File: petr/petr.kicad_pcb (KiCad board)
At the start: 2 copper layers, 38.5 x 53.6 mm, 4 parts

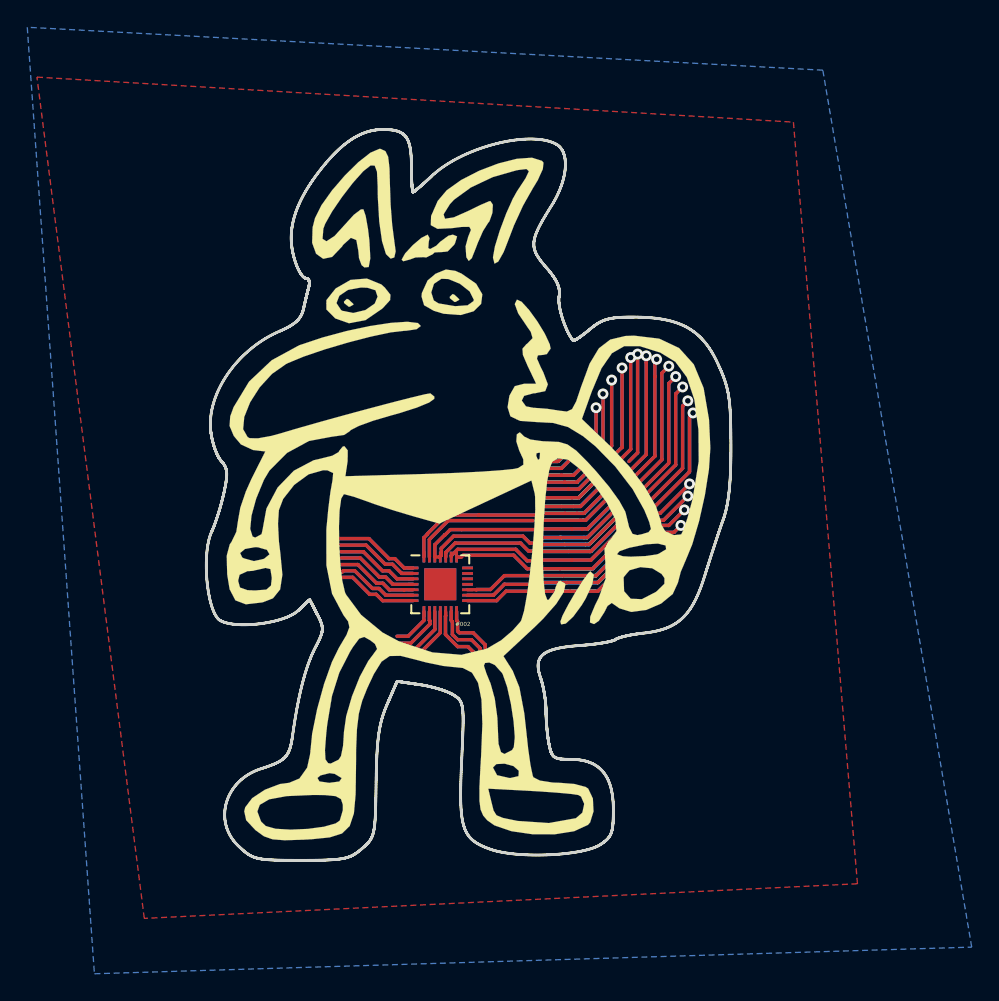
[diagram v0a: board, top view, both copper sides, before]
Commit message: update
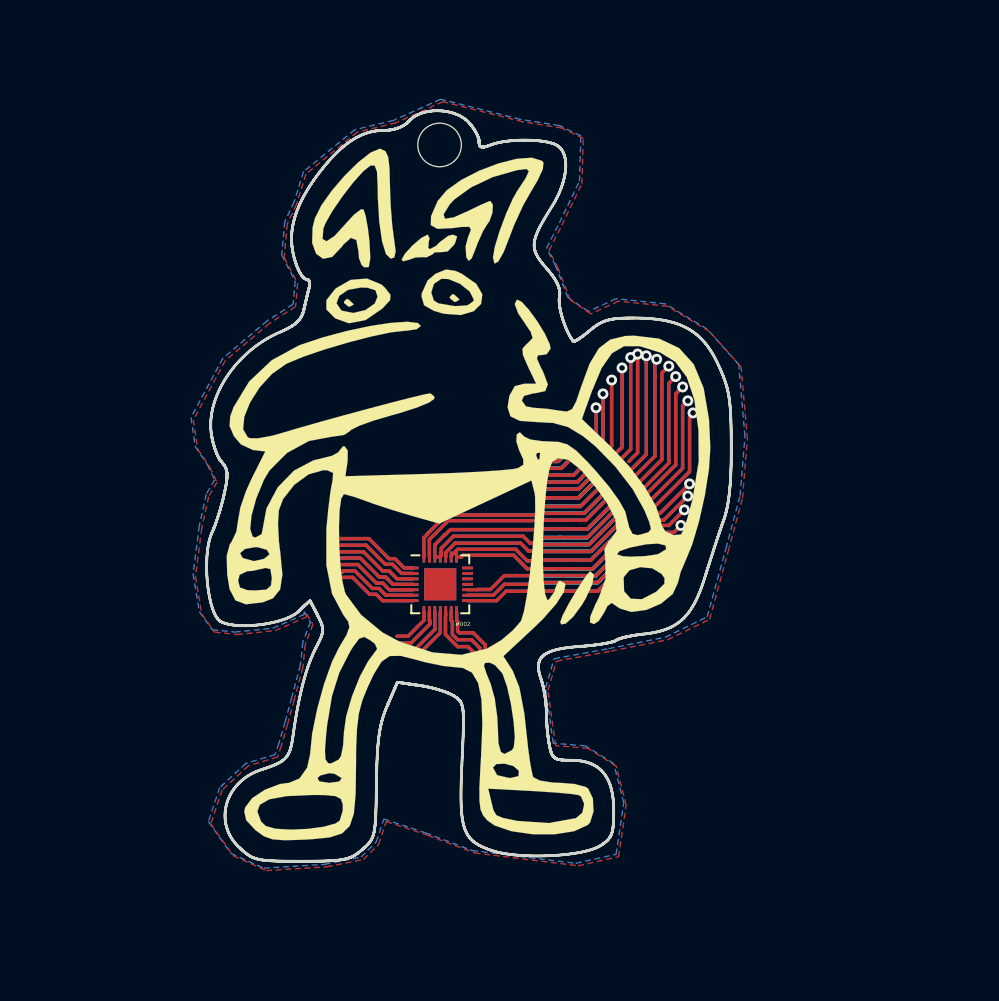
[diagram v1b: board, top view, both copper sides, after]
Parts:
- added REF**: MountingHole_3.2mm_M3, MountingHole:MountingHole_3.2mm_M3, F.Cu at (158.4, 59.6)
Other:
- board size 38.5 x 53.6 mm -> 38.5 x 55.1 mm
